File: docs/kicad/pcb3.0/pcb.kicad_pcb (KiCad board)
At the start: 2 copper layers, 76.2 x 69.8 mm, 22 parts, among them J1 power, J2 coil1, J3 coil2, J4 hall, J5 Sens1, J6 Sens2, J7 Opto, J8 leds, SW1 SW, SW2 SW, U1 L293D, U2 ESP32_DEV_0

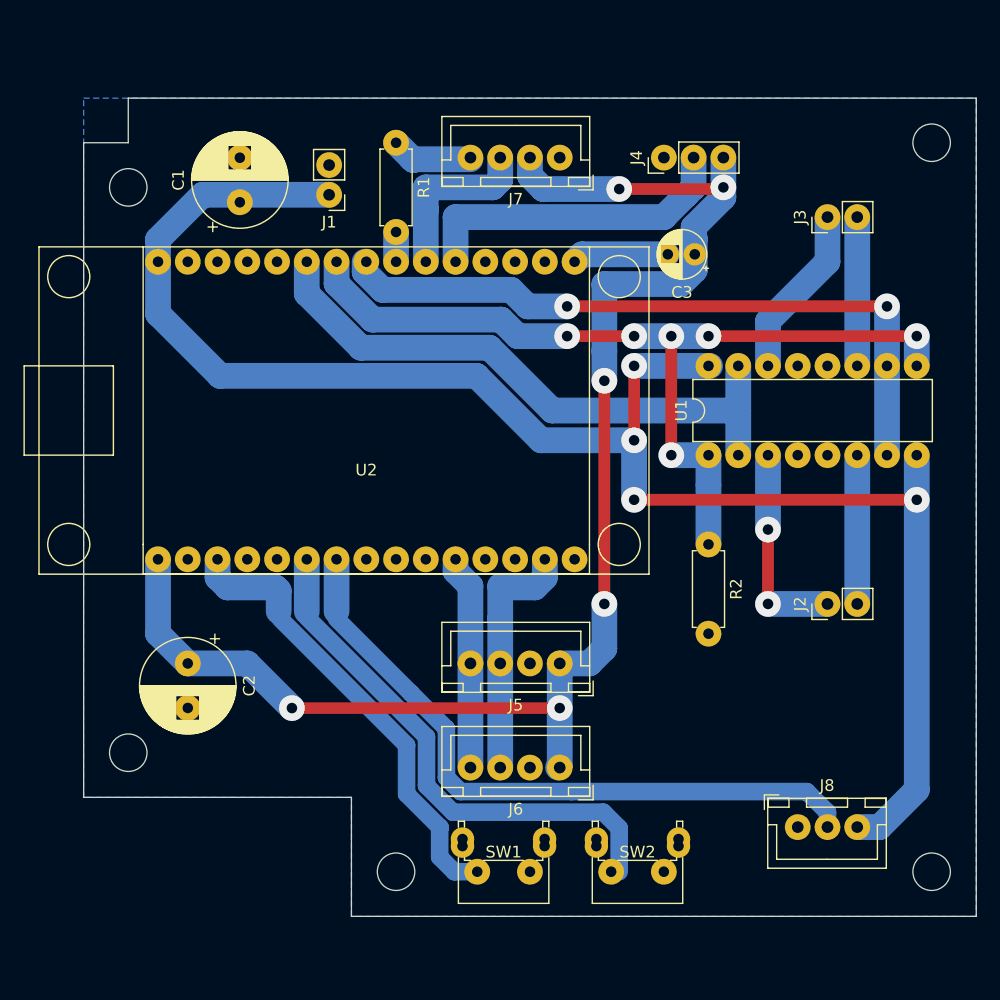
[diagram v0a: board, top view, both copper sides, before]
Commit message: create and build circuit board
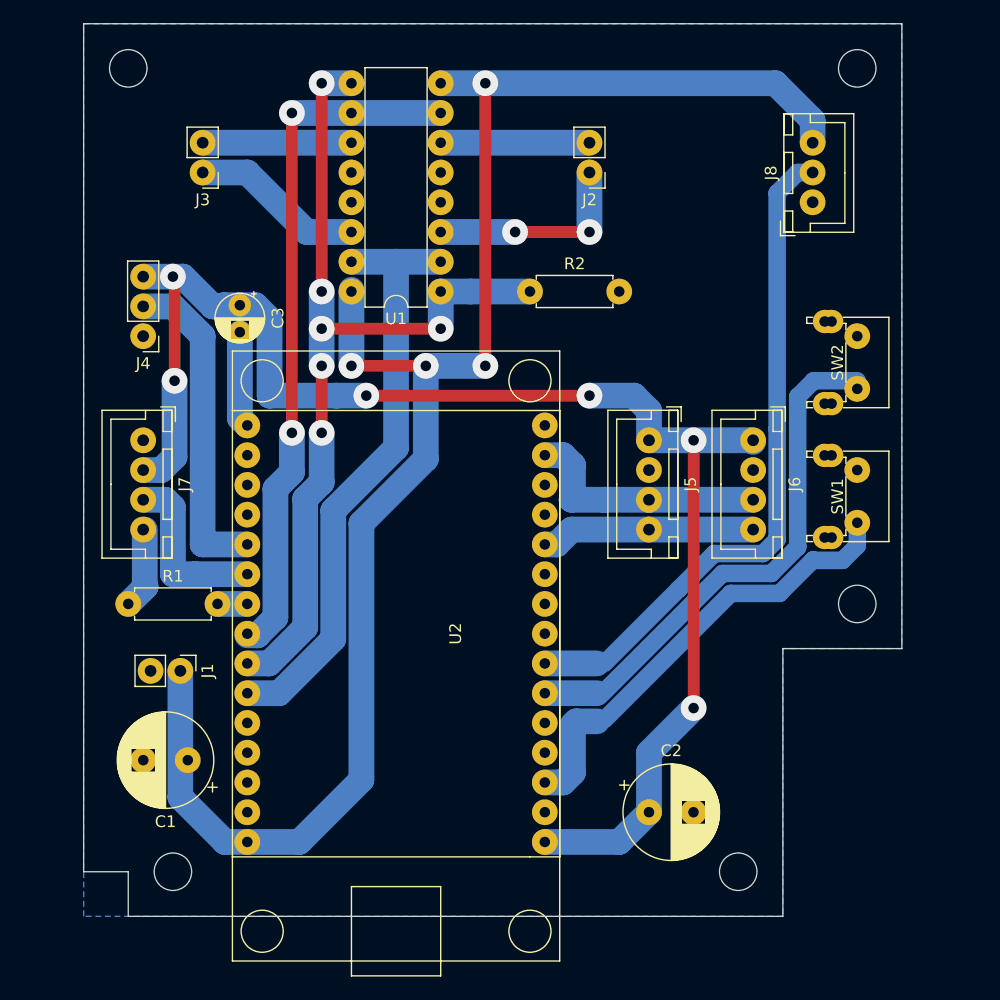
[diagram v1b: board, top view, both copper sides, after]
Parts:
- removed the REF** at (3.81, -14.0)
- removed the REF** at (3.81, -62.2)
- removed the REF** at (26.7, -3.81)
- removed the REF** at (72.4, -3.81)
- added REF**: myMountingHole_3.2mm_M3, 0_my_footprints:myMountingHole_3.2mm_M3, F.Cu at (55.9, -3.81)
- added REF**: myMountingHole_3.2mm_M3, 0_my_footprints:myMountingHole_3.2mm_M3, F.Cu at (7.62, -3.81)
- added REF**: myMountingHole_3.2mm_M3, 0_my_footprints:myMountingHole_3.2mm_M3, F.Cu at (66.0, -26.7)
- added REF**: myMountingHole_3.2mm_M3, 0_my_footprints:myMountingHole_3.2mm_M3, F.Cu at (66.0, -72.4)
- moved REF** 68.9 mm to (3.81, -72.4), turned to 90 degrees
- moved J3 53.5 mm to (10.2, -63.5), turned to 180 degrees
- moved J8 53.4 mm to (62.2, -61.0), turned to 90 degrees
- moved SW2 48.6 mm to (66.0, -49.5), turned to 270 degrees
- moved C1 47.8 mm to (8.89, -13.3), turned to 180 degrees
- moved J4 47.0 mm to (5.08, -49.5), turned to 180 degrees
- moved R1 45.5 mm to (3.81, -26.7), turned to 0 degrees
- moved SW1 44.2 mm to (66.0, -38.1), turned to 270 degrees
- moved J7 43.0 mm to (5.08, -40.6), turned to 270 degrees
- moved J1 42.6 mm to (8.26, -21.0), turned to 270 degrees
- moved J2 42.1 mm to (43.2, -63.5), turned to 180 degrees
- moved C2 41.4 mm to (48.3, -8.89), turned to 0 degrees
- moved C3 39.0 mm to (13.3, -52.1), turned to 270 degrees
- moved J6 32.5 mm to (57.1, -40.6), turned to 270 degrees
- moved U1 26.8 mm to (30.5, -53.3), turned to 180 degrees
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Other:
- board size 76.2 x 69.8 mm -> 69.8 x 76.2 mm
